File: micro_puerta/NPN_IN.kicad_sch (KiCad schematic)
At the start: 6 parts, among them U4 LTV-357T, U7 LTV-357T

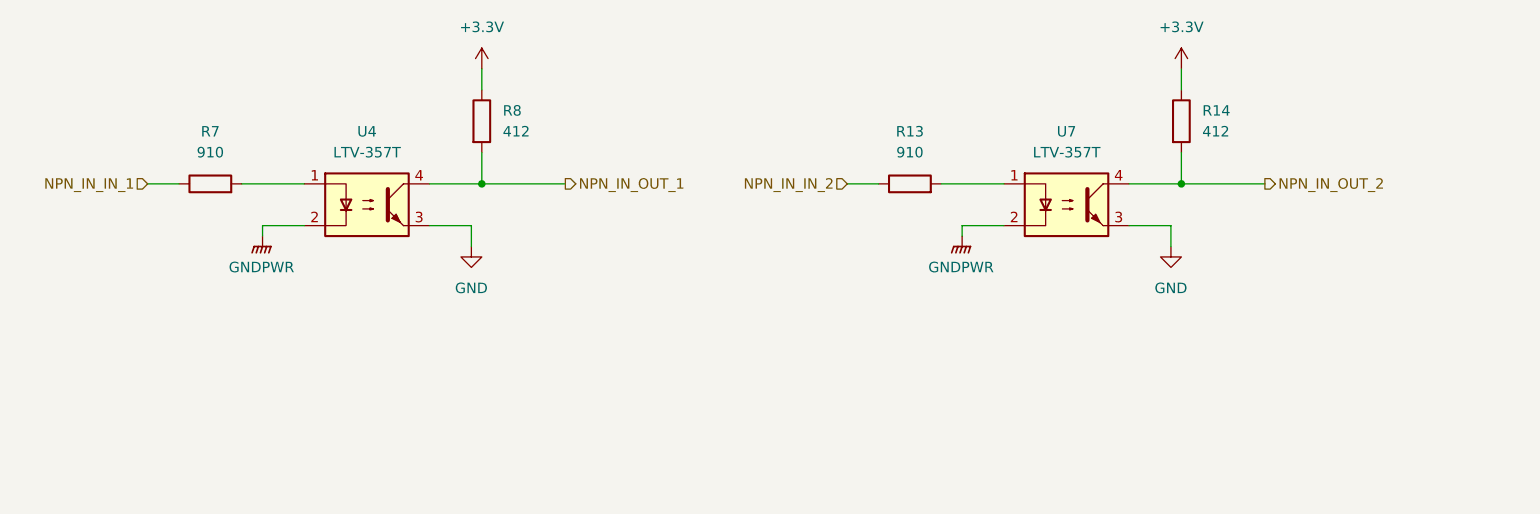
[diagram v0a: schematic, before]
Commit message: Actualizacion 4 de proyecto
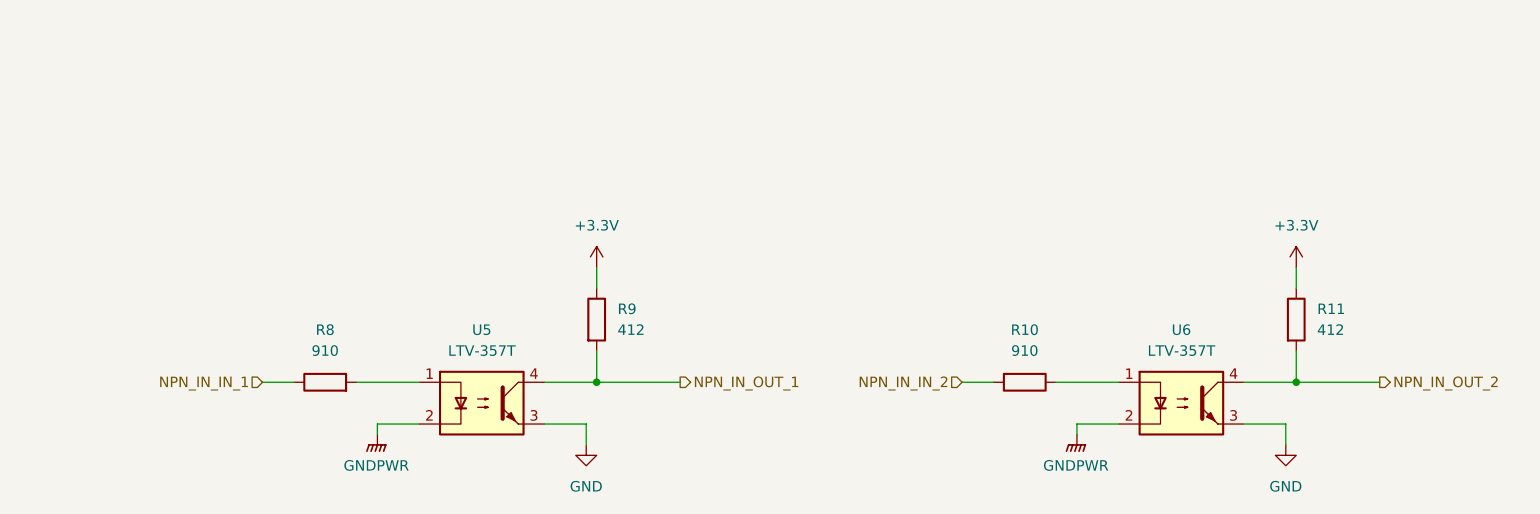
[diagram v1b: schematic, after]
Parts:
- removed R13, R7: 910, symbol Device:R
- removed R14: 412, symbol Device:R
- removed U4, U7: LTV-357T, Package_SO:SO-4_4.4x3.6mm_P2.54mm, symbol Isolator:LTV-357T
- added R10: 910, Resistor_SMD:R_0201_0603Metric, symbol Device:R
- added R11, R9: 412, Resistor_SMD:R_0201_0603Metric, symbol Device:R
- added U5, U6: LTV-357T, Package_SO:SO-4_4.4x3.6mm_P2.54mm, symbol Isolator:LTV-357T
- R8: value 412 -> 910; footprint (none) -> Resistor_SMD:R_0201_0603Metric
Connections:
- net +3.3V: now also R11.1, R9.1; no longer R8.1
- net GND: now also U5.3, U6.3
- net GNDPWR: now also U5.2, U6.2
- net NPN_IN_IN_1: now also R8.1
- net NPN_IN_IN_2: now also R10.2
- net NPN_IN_OUT_1: now also R9.2, U5.4; no longer R8.2
- net NPN_IN_OUT_2: now also R11.2, U6.4
- new net: R10.1, U6.1
- new net: R8.2, U5.1
